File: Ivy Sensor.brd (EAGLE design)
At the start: 67.9 x 47 mm, 19 parts, among them Q1 C1815, SW1 OS102011MA1Q

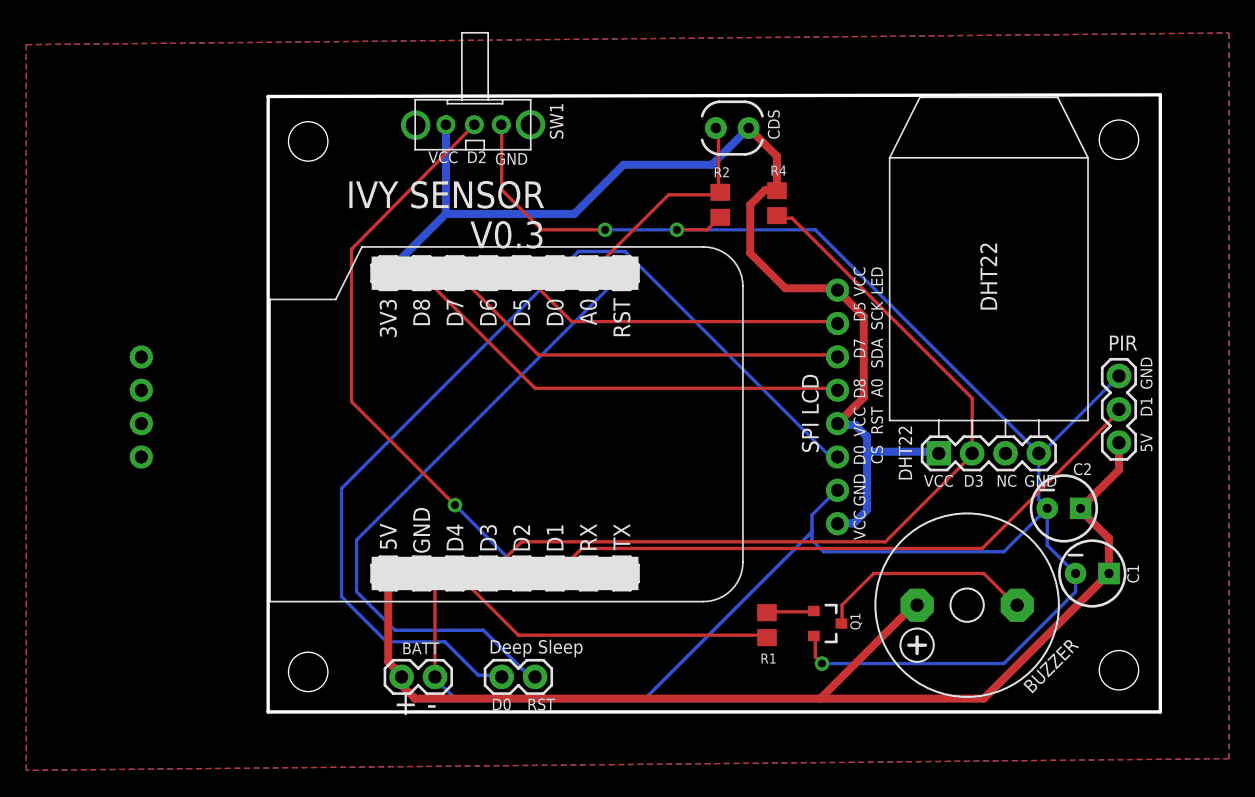
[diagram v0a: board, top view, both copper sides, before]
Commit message: Update design to version 0.4
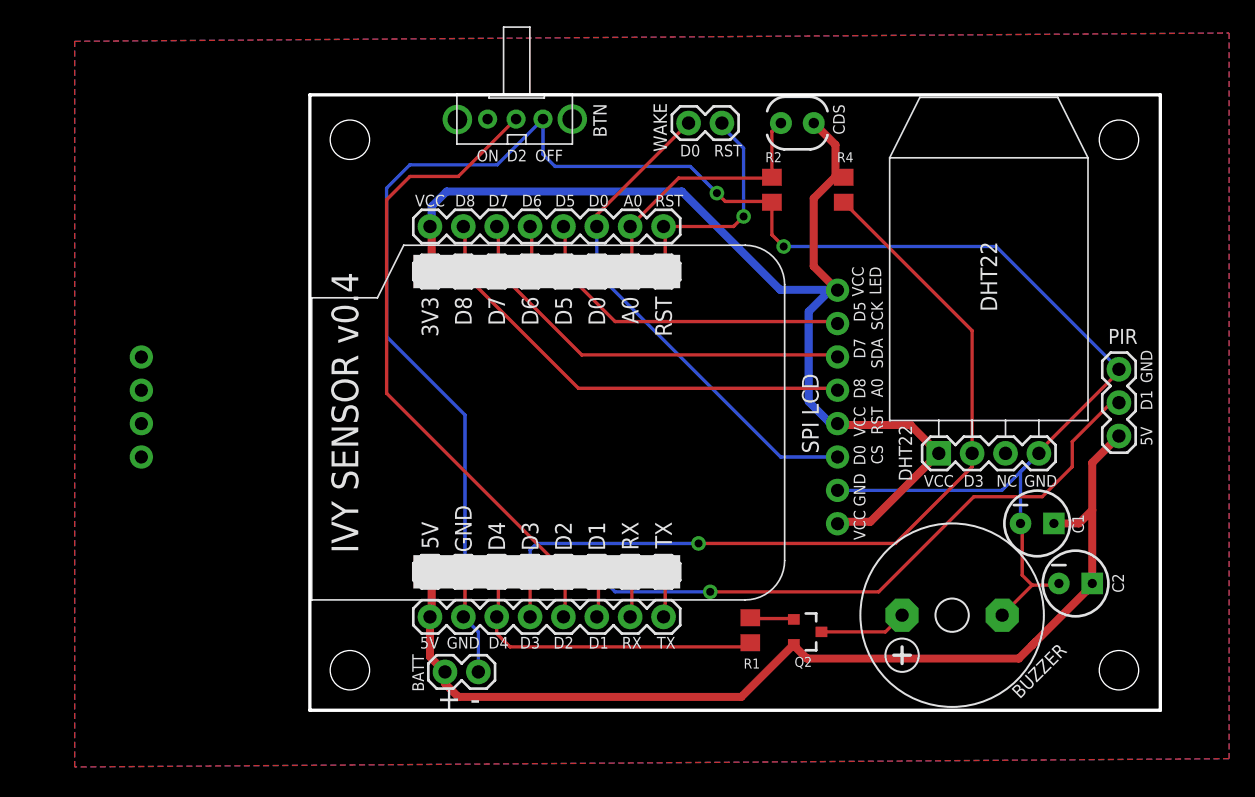
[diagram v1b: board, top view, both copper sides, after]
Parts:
- removed Q1: C1815, SparkFun-DiscreteSemi:SOT23-3
- removed SW1: OS102011MA1Q, adafruit:OS102011MA1Q
- added BTN: OS102011MA1Q, adafruit:OS102011MA1Q
- added JP1, JP2: (no value), SparkFun-Connectors:1X08_ROUND
- added Q2: A1015, SparkFun-DiscreteSemi:SOT23-3
- C1: value 47uF/16V -> 47uF
- moved DEEP_SLEEP_JP 44.5 mm to (52.6, 49.1)
- moved C2 5.78 mm to (79.5, 14.1)
- moved C1 5.66 mm to (76.6, 18.7)
- moved R4 5.18 mm to (61.8, 44.1)
- moved R3 4.97 mm to (58.4, 49.1)
- moved R2 4.10 mm to (56.4, 44.1)
- moved BATT 3.32 mm to (34.0, 7.37)
- moved U$6 3.18 mm to (24.3, 7.49)
- moved U$2 3.18 mm to (30.4, 37.8)
- moved U$9 3.18 mm to (24.3, 47.9)
- moved BUZZER 1.37 mm to (70.1, 11.7)
- moved R1 1.33 mm to (54.7, 10.5)
- moved PIR 0.51 mm to (82.8, 25.3)
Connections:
- removed net N$1: BUZZER.-, Q1.3
- removed net N$3: Q1.1, R1.1
- new net RX: JP2.2, U$2.RX
- new net TX: JP2.1, U$2.TX
- new net T_B: Q2.1, R1.1
- new net T_C: BUZZER.+, Q2.3
- net 5V: now also JP2.8, Q2.2; no longer BUZZER.+
- net A0: now also JP1.7
- net D0: now also JP1.6
- net D1: now also JP2.3
- net D2: now also BTN.2, JP2.4; no longer SW1.2
- net D3: now also JP2.5
- net D4: now also JP2.6
- net D5: now also JP1.5
- net D6: now also JP1.4
- net D7: now also JP1.3
- net D8: now also JP1.2
- net GND: now also BTN.1, BUZZER.-, JP2.7; no longer Q1.2, SW1.1
- net RST: now also JP1.8
- net VCC: now also JP1.1; no longer SW1.3
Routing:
- net D0: track 74.8 -> 38.4 mm
- net RST: track 48.8 -> 17.9 mm, vias 0 -> 1
- net GND: track 169.9 -> 150.6 mm, vias 3 -> 2
- net N$1: track 16.7 -> 0.00 mm
- net 5V: track 89.6 -> 79.1 mm
- net T_C: track 0.00 -> 6.67 mm
- net D2: track 43.2 -> 49.8 mm, vias 1 -> 0
- net D6: track 0.00 -> 3.66 mm
- net RX: track 0.00 -> 3.66 mm
- net N$3: track 3.60 -> 0.00 mm
- net TX: track 0.00 -> 3.41 mm
- net T_B: track 0.00 -> 3.35 mm
- net D1: track 48.3 -> 50.9 mm, vias 0 -> 1
- net A0: track 17.7 -> 20.2 mm
- net VCC: track 87.0 -> 85.6 mm
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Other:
- board size 67.9 x 47 mm -> 64.7 x 46.9 mm
- board text added: "A0"
- board text added: "D4"
- board text added: "D5"
- board text added: "D6"
- board text added: "D7"
- board text added: "D8"
- board text added: "IVY SENSOR v0.4"
- board text added: "OFF"
- board text added: "ON"
- board text added: "RX"
- board text added: "TX"
- board text added: "WAKE"
- board text removed: "Deep Sleep"
- board text removed: "IVY SENSOR V0.3"
